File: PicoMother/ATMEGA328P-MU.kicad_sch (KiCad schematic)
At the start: 15 parts, among them J3 M20-9980345, SW1 SW_Push, U4 ATMEGA328P-MU, Y1 CSTNE16M0V530000R0

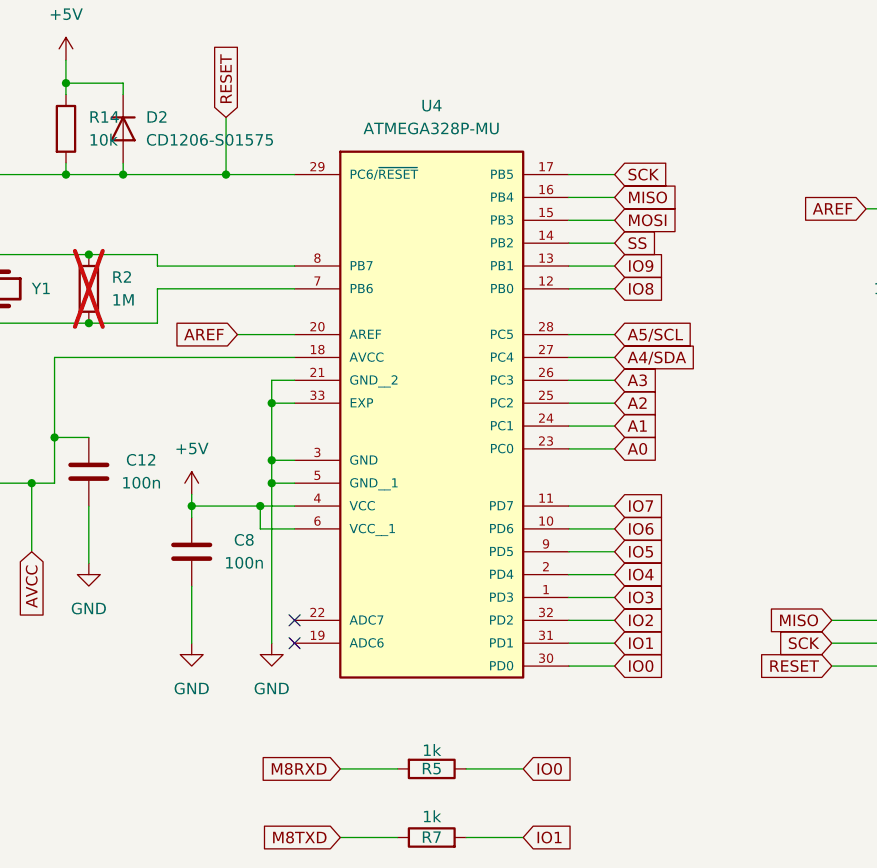
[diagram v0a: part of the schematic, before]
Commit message: avancement schema
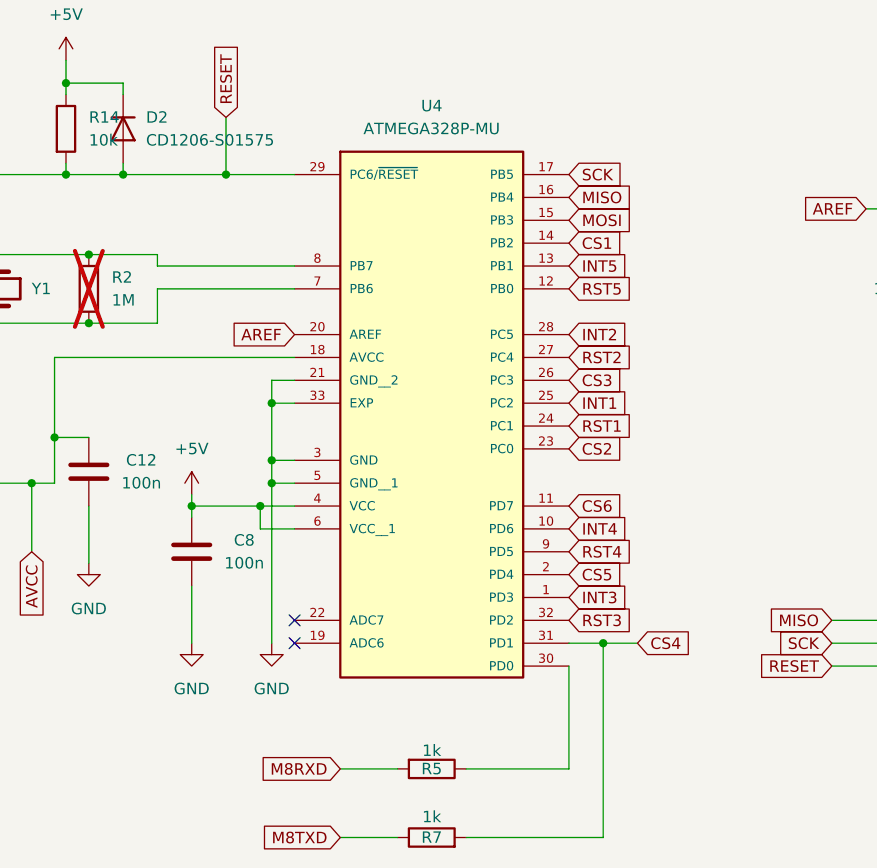
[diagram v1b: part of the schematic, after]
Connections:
- net A0 renamed CS2
- net A1 renamed RST1
- net A2 renamed INT1
- net A3 renamed CS3
- net A4/SDA renamed RST2
- net A5/SCL renamed INT2
- net IO0: no longer names the net of R5.1, U4.30 (PD0)
- net IO1 renamed CS4
- net IO2 renamed RST3
- net IO3 renamed INT3
- net IO4 renamed CS5
- net IO5 renamed RST4
- net IO6 renamed INT4
- net IO7 renamed CS6
- net IO8 renamed RST5
- net IO9 renamed INT5
- net SS renamed CS1

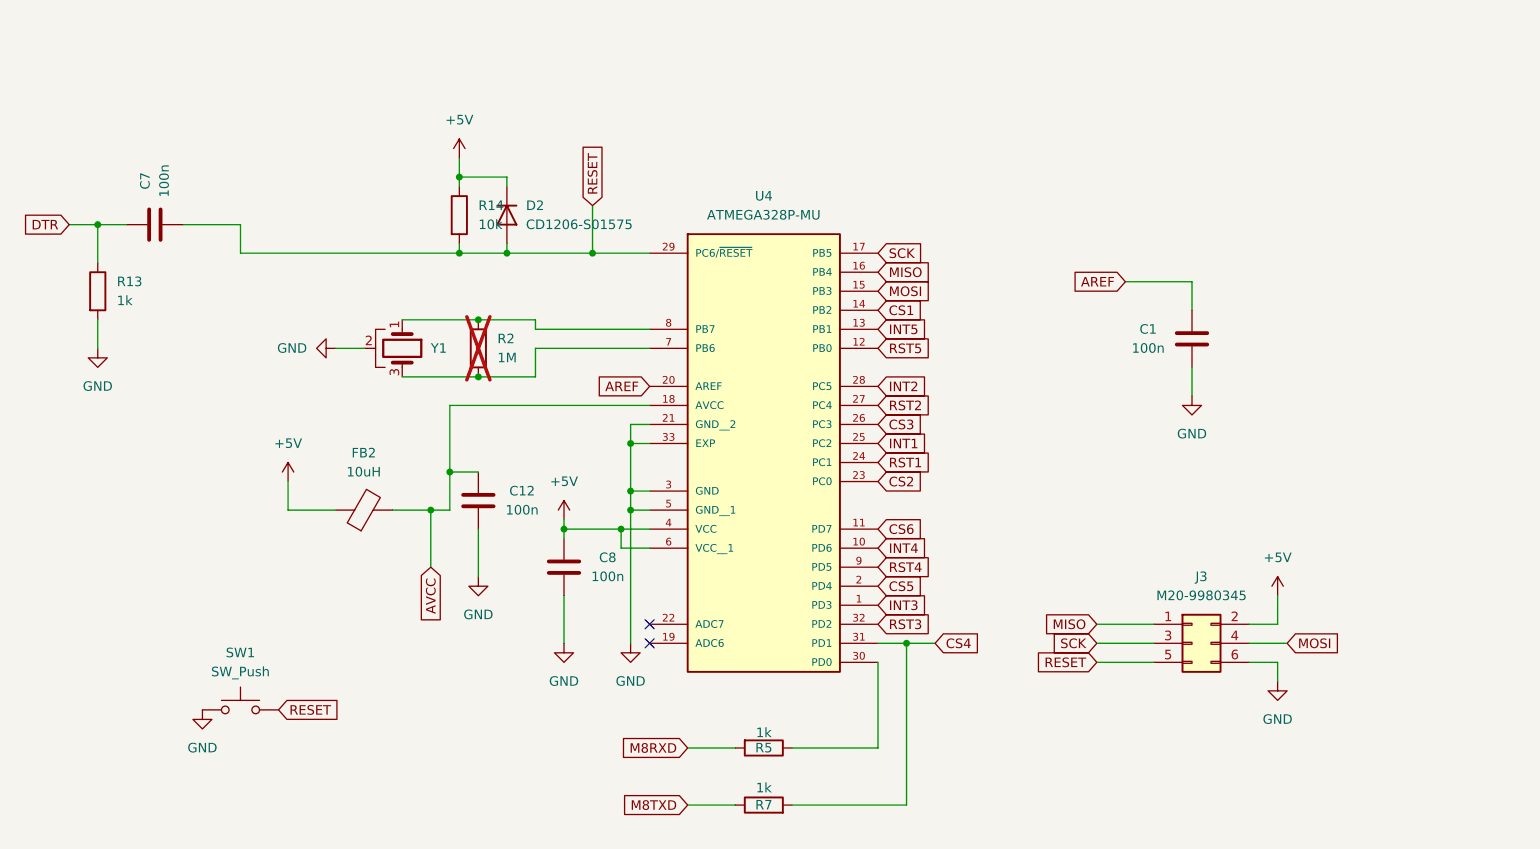
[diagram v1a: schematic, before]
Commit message: Schema PicoMother
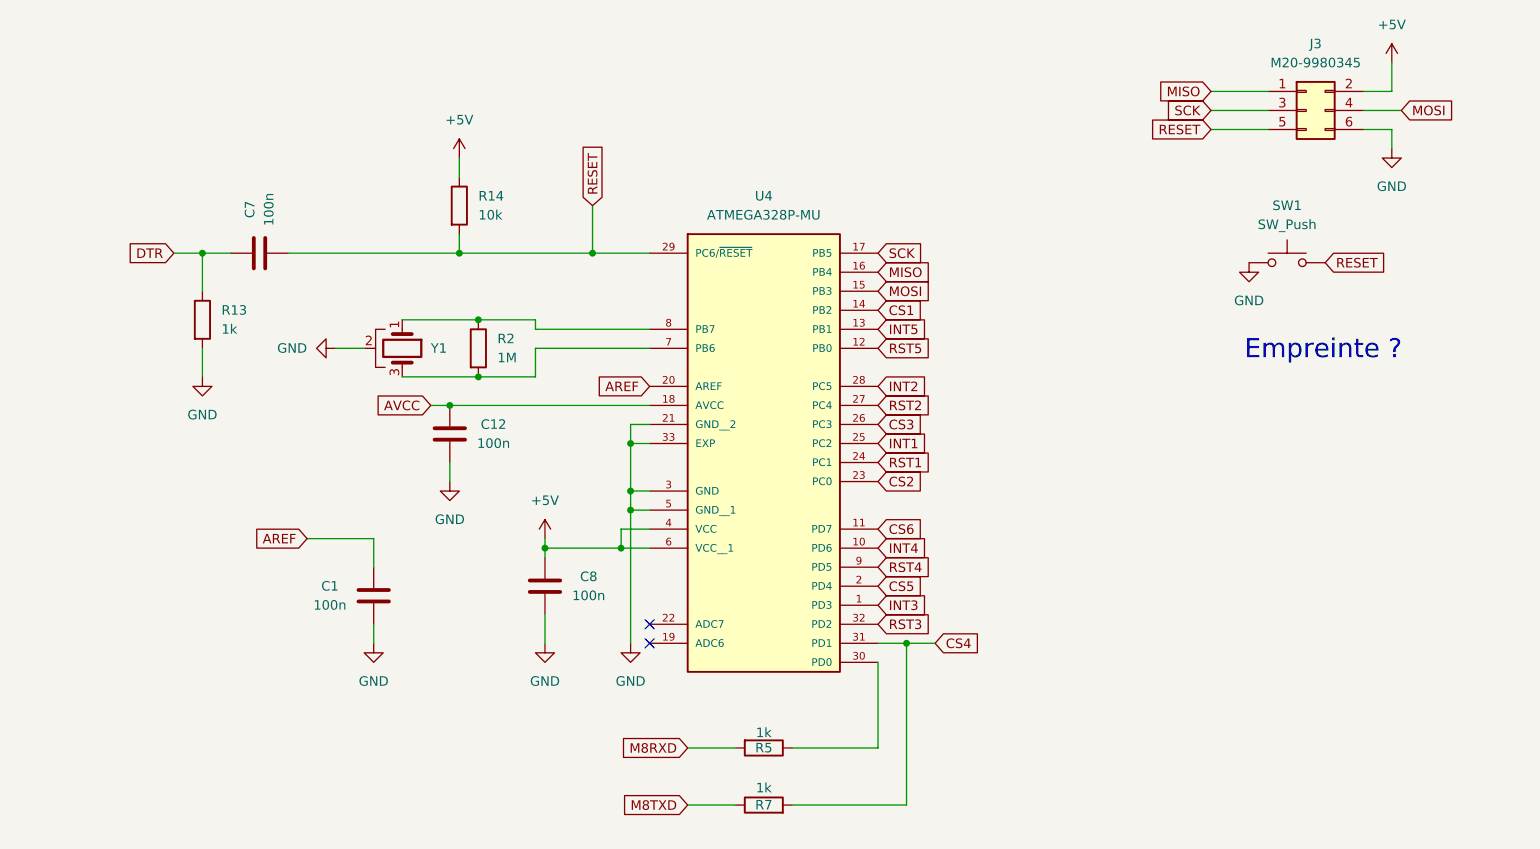
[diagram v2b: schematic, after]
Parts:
- removed D2: CD1206-S01575, Diode_SMD:D_1206_3216Metric, symbol Device:D
- removed FB2: 10uH, Inductor_SMD:L_0805_2012Metric, symbol Device:FerriteBead
- C1, C12, C7, C8: footprint Capacitor_SMD:C_0603_1608Metric -> Capacitor_SMD:C_0603_1608Metric_Pad1.08x0.95mm_HandSolder
- R2: footprint Resistor_SMD:R_0603_1608Metric -> Resistor_SMD:R_0603_1608Metric_Pad0.98x0.95mm_HandSolder; now fitted
- Y1: value CSTNE16M0V530000R0 -> 16Mhz; footprint Crystal:Resonator_SMD_Murata_CSTxExxV-3Pin_3.0x1.1mm -> Crystal:Crystal_SMD_SeikoEpson_FA238-4Pin_3.2x2.5mm_HandSoldering
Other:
- note added: "Empreinte ?"
- moved on the sheet: C1, C12, C7, C8, J3, R13, R14, SW1

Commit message: Premier Schema
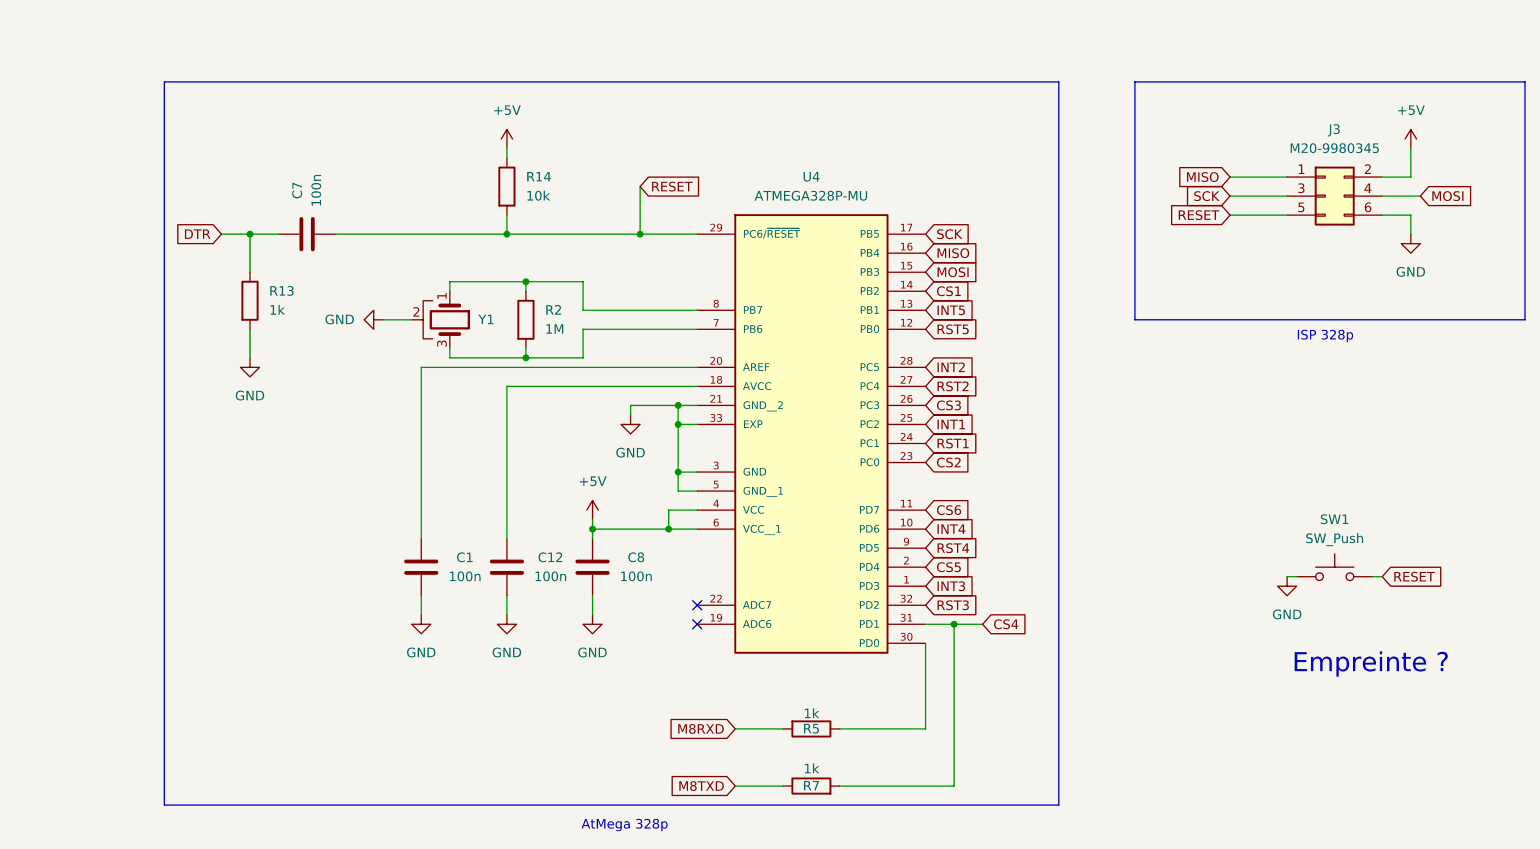
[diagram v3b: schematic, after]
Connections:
- net AREF: no longer names the net of C1.1, U4.20 (AREF)
- net AVCC: no longer names the net of C12.1, U4.18 (AVCC)
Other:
- note added: "AtMega 328p"
- note added: "ISP 328p"
- moved on the sheet: C1, C12, C7, C8, J3, R13, R14, R2, R5, R7, SW1, U4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

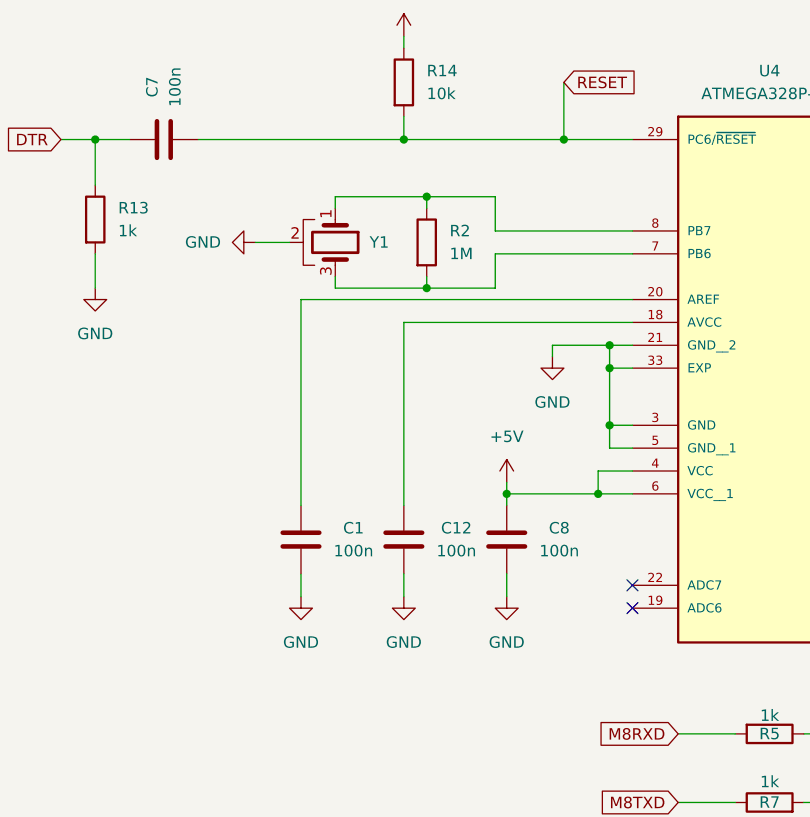
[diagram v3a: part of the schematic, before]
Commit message: correction schematique quartz
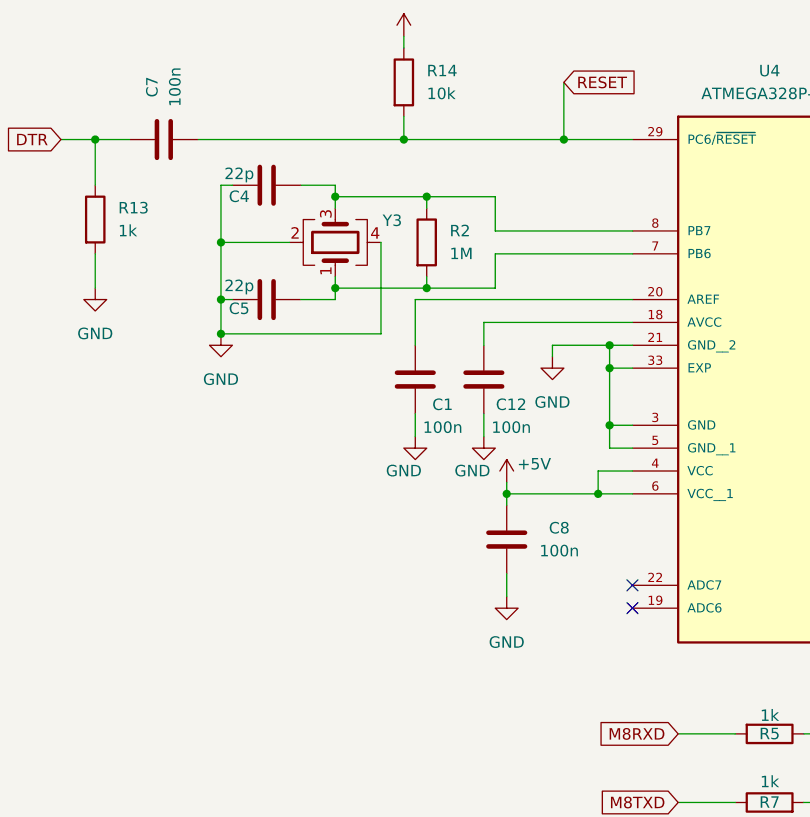
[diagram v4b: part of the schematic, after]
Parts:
- removed Y1: 16Mhz, Crystal:Crystal_SMD_SeikoEpson_FA238-4Pin_3.2x2.5mm_HandSoldering, symbol Device:Crystal_GND2
- added C4, C5: 22p, Capacitor_SMD:C_0603_1608Metric_Pad1.08x0.95mm_HandSolder, symbol Device:C
- added Y3: Crystal_GND24, Crystal:Crystal_SMD_SeikoEpson_FA238-4Pin_3.2x2.5mm_HandSoldering, symbol Device:Crystal_GND24
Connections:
- net GND: now also C4.2, C5.2, Y3.2, Y3.4
- net at R2.1, U4.8 (PB7): now also C4.1, Y3.3
- net at R2.2, U4.7 (PB6): now also C5.1, Y3.1
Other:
- moved on the sheet: C1, C12
